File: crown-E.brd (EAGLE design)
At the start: 57.8 x 50.8 mm, 85 parts

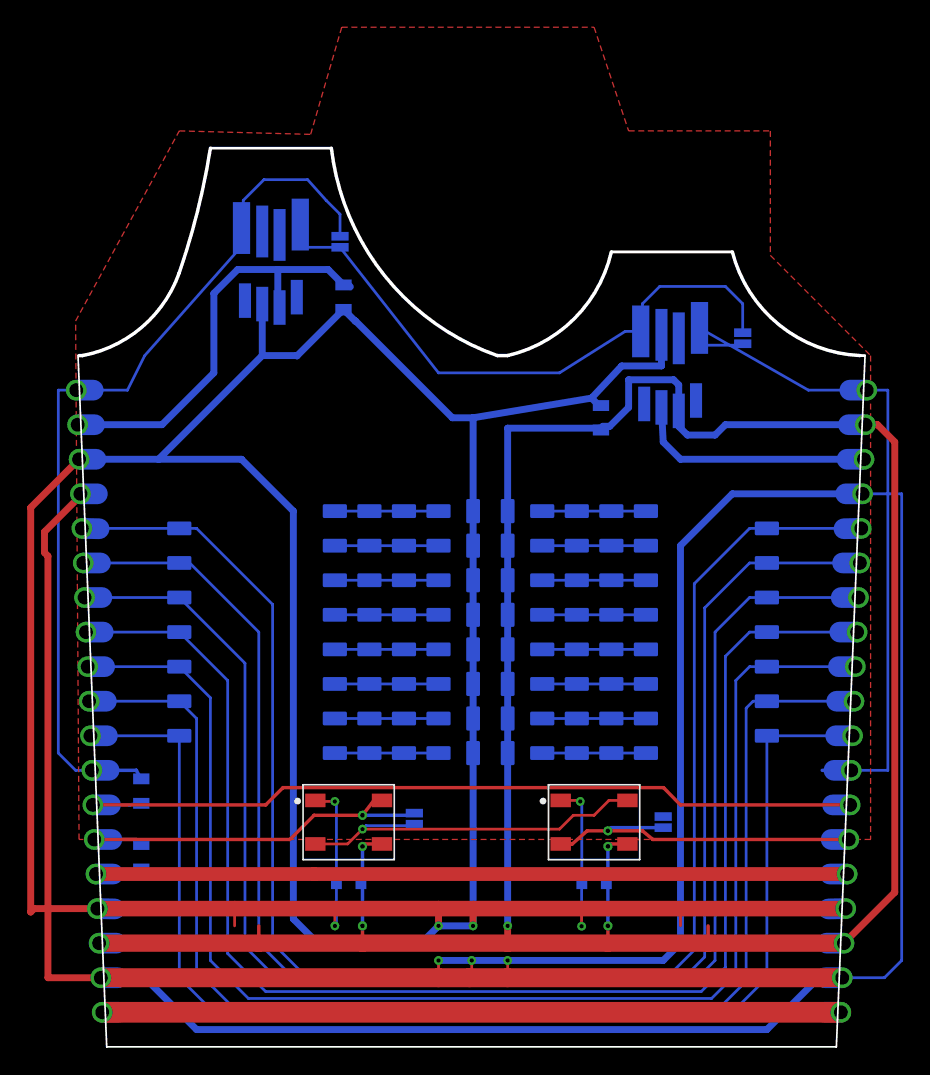
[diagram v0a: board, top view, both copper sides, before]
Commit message: tidied up a little bit
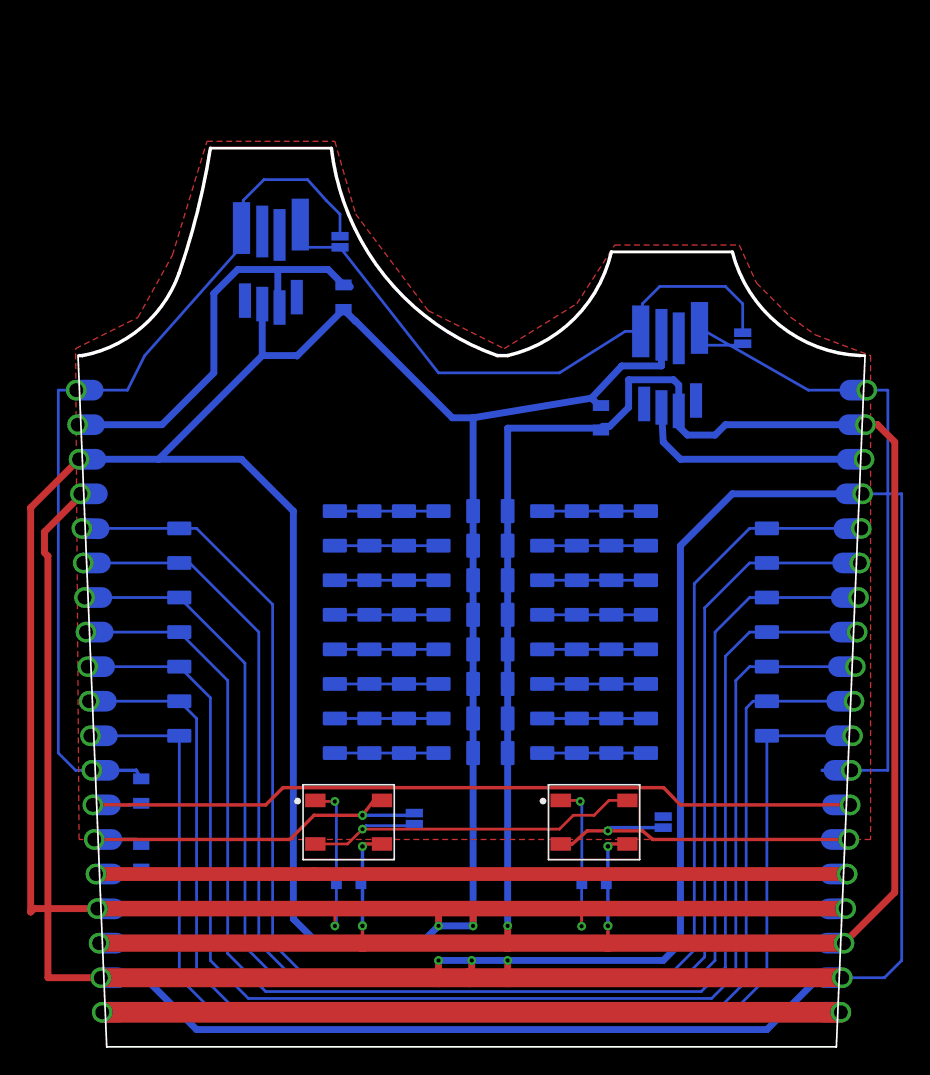
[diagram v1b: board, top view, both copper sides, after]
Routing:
- net VLIVE: track 294.3 -> 291.8 mm
- net GND: track 218.2 -> 215.7 mm
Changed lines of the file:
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@@
 <grid distance="10" unitdist="mil" unit="mil" style="lines" multiple="5" display="yes" altdistance="1" altunitdist="mil" altunit="mil"/>
 <layers>
-<layer number="1" name="Top" color="4" fill="1" visible="no" active="yes"/>
-<layer number="16" name="Bottom" color="1" fill="1" visible="no" active="yes"/>
-<layer number="17" name="Pads" color="2" fill="1" visible="no" active="yes"/>
-<layer number="18" name="Vias" color="2" fill="1" visible="no" active="yes"/>
-<layer number="19" name="Unrouted" color="6" fill="1" visible="no" active="yes"/>
+<layer number="1" name="Top" color="4" fill="1" visible="yes" active="yes"/>
+<layer number="16" name="Bottom" color="1" fill="1" visible="yes" active="yes"/>
+<layer number="17" name="Pads" color="2" fill="1" visible="yes" active="yes"/>
+<layer number="18" name="Vias" color="2" fill="1" visible="yes" active="yes"/>
+<layer number="19" name="Unrouted" color="6" fill="1" visible="yes" active="yes"/>
 <layer number="20" name="Dimension" color="15" fill="1" visible="yes" active="yes"/>
-<layer number="21" name="tPlace" color="16" fill="1" visible="no" active="yes"/>
-<layer number="22" name="bPlace" color="14" fill="1" visible="no" active="yes"/>
-<layer number="23" name="tOrigins" color="15" fill="1" visible="no" active="yes"/>
-<layer number="24" name="bOrigins" color="15" fill="1" visible="no" active="yes"/>
+<layer number="21" name="tPlace" color="16" fill="1" visible="yes" active="yes"/>
+<layer number="22" name="bPlace" color="14" fill="1" visible="yes" active="yes"/>
+<layer number="23" name="tOrigins" color="15" fill="1" visible="yes" active="yes"/>
+<layer number="24" name="bOrigins" color="15" fill="1" visible="yes" active="yes"/>
 <layer number="25" name="tNames" color="7" fill="1" visible="no" active="yes"/>
 <layer number="26" name="bNames" color="7" fill="1" visible="no" active="yes"/>
@@
 <layer number="28" name="bValues" color="7" fill="1" visible="no" active="yes"/>
 <layer number="29" name="tStop" color="7" fill="3" visible="yes" active="yes"/>
-<layer number="30" name="bStop" color="7" fill="6" visible="no" active="yes"/>
+<layer number="30" name="bStop" color="7" fill="6" visible="yes" active="yes"/>
 <layer number="31" name="tCream" color="7" fill="4" visible="no" active="yes"/>
 <layer number="32" name="bCream" color="7" fill="5" visible="no" active="yes"/>
@@
 <layer number="43" name="vRestrict" color="2" fill="10" visible="no" active="yes"/>
 <layer number="44" name="Drills" color="7" fill="1" visible="no" active="yes"/>
-<layer number="45" name="Holes" color="7" fill="1" visible="no" active="yes"/>
+<layer number="45" name="Holes" color="7" fill="1" visible="yes" active="yes"/>
 <layer number="46" name="Milling" color="3" fill="1" visible="no" active="yes"/>
 <layer number="47" name="Measures" color="7" fill="1" visible="no" active="yes"/>
@@
 <layer number="49" name="Reference" color="7" fill="1" visible="no" active="yes"/>
 <layer number="50" name="dxf" color="7" fill="1" visible="no" active="no"/>
-<layer number="51" name="tDocu" color="6" fill="1" visible="no" active="yes"/>
+<layer number="51" name="tDocu" color="6" fill="1" visible="yes" active="yes"/>
 <layer number="52" name="bDocu" color="7" fill="1" visible="no" active="yes"/>
 <layer number="53" name="tGND_GNDA" color="7" fill="9" visible="no" active="no"/>
@@
 <contactref element="PTH1" pad="P$2"/>
 <contactref element="PTH1" pad="P$6"/>
-<wire x1="1.778" y1="7.62" x2="13.462" y2="7.62" width="1.27" layer="1"/>
+<wire x1="1.778" y1="7.62" x2="21.082" y2="7.62" width="1.27" layer="1"/>
 <contactref element="SMD2" pad="3"/>
 <contactref element="C2" pad="2"/>
@@
 <contactref element="C3" pad="2"/>
 <contactref element="C4" pad="2"/>
-<wire x1="13.462" y1="7.62" x2="21.082" y2="7.62" width="1.27" layer="1"/>
 <wire x1="21.082" y1="7.62" x2="31.75" y2="7.62" width="1.27" layer="1"/>
 <wire x1="31.75" y1="7.62" x2="39.116" y2="7.62" width="1.27" layer="1"/>
-<wire x1="39.116" y1="7.62" x2="46.482" y2="7.62" width="1.27" layer="1"/>
-<wire x1="46.482" y1="7.62" x2="56.4642" y2="7.62" width="1.27" layer="1"/>
+<wire x1="39.116" y1="7.62" x2="56.4642" y2="7.62" width="1.27" layer="1"/>
 <wire x1="22.516" y1="14.91" x2="21.26" y2="14.91" width="0.254" layer="1"/>
 <wire x1="21.26" y1="14.91" x2="21.082" y2="14.732" width="0.254" layer="1"/>
@@
 <wire x1="39.116" y1="12.192" x2="39.116" y2="8.89" width="0.254" layer="16"/>
 <wire x1="39" y1="12.192" x2="39.116" y2="12.192" width="0.254" layer="16"/>
-<wire x1="46.482" y1="8.89" x2="46.482" y2="7.62" width="0.254" layer="1"/>
 <via x="39.116" y="8.89" extent="1-16" drill="0.3302"/>
 <wire x1="39.116" y1="8.89" x2="39.116" y2="7.62" width="0.254" layer="1"/>
 <via x="21.082" y="8.89" extent="1-16" drill="0.3302"/>
 <wire x1="21.082" y1="8.89" x2="21.082" y2="7.62" width="0.254" layer="1"/>
-<wire x1="13.462" y1="8.89" x2="13.462" y2="7.62" width="0.254" layer="1"/>
 <via x="31.75" y="8.89" extent="1-16" drill="0.3048"/>
 <wire x1="31.75" y1="8.89" x2="31.75" y2="7.62" width="0.508" layer="1"/>
@@
 <polygon width="0.2032" layer="1" isolate="0.254" orphans="yes">
 <vertex x="0.254" y="15.24"/>
-<vertex x="0" y="53.34"/>
-<vertex x="7.62" y="67.31"/>
-<vertex x="17.272" y="67.056"/>
-<vertex x="19.558" y="74.93"/>
-<vertex x="38.1" y="74.93"/>
-<vertex x="40.64" y="67.31"/>
-<vertex x="51.054" y="67.31"/>
-<vertex x="51.054" y="58.166"/>
+<vertex x="0" y="51.308"/>
+<vertex x="4.572" y="53.594"/>
+<vertex x="7.112" y="58.166"/>
+<vertex x="9.652" y="66.548"/>
+<vertex x="19.05" y="66.548"/>
+<vertex x="20.574" y="61.214"/>
+<vertex x="25.908" y="54.102"/>
+<vertex x="31.496" y="51.308"/>
+<vertex x="36.83" y="54.61"/>
+<vertex x="39.624" y="58.928"/>
+<vertex x="48.768" y="58.928"/>
+<vertex x="50.038" y="56.134"/>
+<vertex x="52.578" y="53.594"/>
+<vertex x="54.356" y="52.324"/>
 <vertex x="58.42" y="50.8"/>
 <vertex x="58.42" y="15.24"/>
@@
 <contactref element="U$2" pad="P$4"/>
 <contactref element="U$2" pad="P$23"/>
-<wire x1="1.6002" y1="10.16" x2="11.684" y2="10.16" width="1.143" layer="1"/>
+<wire x1="1.6002" y1="10.16" x2="19.05" y2="10.16" width="1.143" layer="1"/>
 <contactref element="SMD1" pad="1"/>
 <contactref element="SMD2" pad="1"/>
@@
 <contactref element="C1" pad="1"/>
 <contactref element="C2" pad="1"/>
-<wire x1="11.684" y1="10.16" x2="19.05" y2="10.16" width="1.143" layer="1"/>
 <wire x1="19.05" y1="10.16" x2="26.67" y2="10.16" width="1.143" layer="1"/>
 <wire x1="26.67" y1="10.16" x2="29.21" y2="10.16" width="1.143" layer="1"/>
 <wire x1="29.21" y1="10.16" x2="37.1856" y2="10.16" width="1.143" layer="1"/>
-<wire x1="37.1856" y1="10.16" x2="44.45" y2="10.16" width="1.143" layer="1"/>
-<wire x1="44.45" y1="10.16" x2="56.5912" y2="10.16" width="1.143" layer="1"/>
-<wire x1="11.684" y1="8.89" x2="11.684" y2="10.16" width="0.2032" layer="1"/>
+<wire x1="37.1856" y1="10.16" x2="56.5912" y2="10.16" width="1.143" layer="1"/>
 <wire x1="19.166" y1="12.192" x2="19.166" y2="8.89" width="0.2032" layer="16"/>
 <wire x1="19.166" y1="8.89" x2="19.05" y2="8.89" width="0.2032" layer="16"/>
@@
 <via x="29.21" y="8.89" extent="1-16" drill="0.3048"/>
 <wire x1="29.21" y1="8.89" x2="29.21" y2="10.16" width="0.508" layer="1"/>
-<wire x1="44.45" y1="8.89" x2="44.45" y2="10.16" width="0.2032" layer="1"/>
 <contactref element="U$2" pad="P$17"/>
 <wire x1="0.254" y1="43.18" x2="6.096" y2="43.18" width="0.508" layer="16"/>
@@
 <wire x1="25.4" y1="7.62" x2="26.67" y2="8.89" width="0.508" layer="16"/>
 <wire x1="26.67" y1="8.89" x2="29.21" y2="8.89" width="0.508" layer="16"/>
+<wire x1="26.67" y1="8.89" x2="26.67" y2="10.16" width="0.508" layer="1"/>
 <wire x1="43.053" y1="50.038" x2="43.053" y2="46.99" width="0" layer="19" extent="16-16"/>
 <wire x1="13.716" y1="59.9186" x2="13.716" y2="54.5846" width="0" layer="19" extent="16-16"/>
-<wire x1="26.67" y1="8.89" x2="26.67" y2="10.16" width="0.508" layer="1"/>
 </signal>
 <signal name="PTH-DO">
@@
 <via x="31.75" y="6.35" extent="1-16" drill="0.3048"/>
 <wire x1="57.912" y1="40.64" x2="57.8358" y2="40.64" width="0.2032" layer="16"/>
-<wire x1="26.67" y1="6.35" x2="26.67" y2="5.08" width="0.2032" layer="1"/>
-<wire x1="31.75" y1="6.35" x2="31.75" y2="5.08" width="0.2032" layer="1"/>
-<wire x1="29.1084" y1="6.35" x2="29.1084" y2="5.2324" width="0.2032" layer="1"/>
+<wire x1="26.67" y1="6.35" x2="26.67" y2="5.08" width="0.508" layer="1"/>
+<wire x1="31.75" y1="6.35" x2="31.75" y2="5.08" width="0.508" layer="1"/>
+<wire x1="29.1084" y1="6.35" x2="29.1084" y2="5.2324" width="0.508" layer="1"/>
 <wire x1="29.1084" y1="5.2324" x2="28.956" y2="5.08" width="0.2032" layer="1"/>
 <wire x1="26.67" y1="6.35" x2="43.18" y2="6.35" width="0.508" layer="16"/>
